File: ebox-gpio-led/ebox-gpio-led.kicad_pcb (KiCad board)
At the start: 2 copper layers, 45 x 75 mm, 26 parts, among them J1 xconch_pinheader_2x40, J2 xconch_pinsocket_2x40

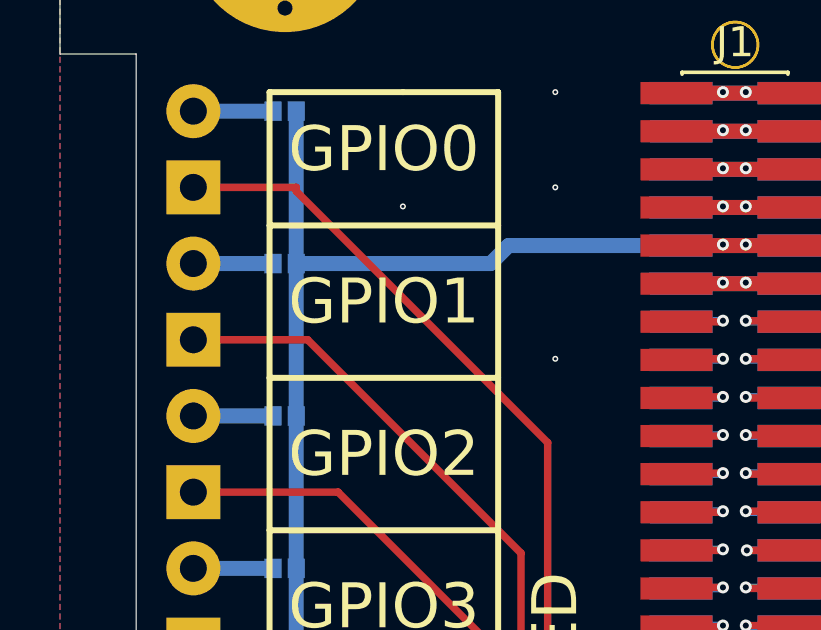
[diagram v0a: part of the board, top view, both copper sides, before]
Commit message: update some documents
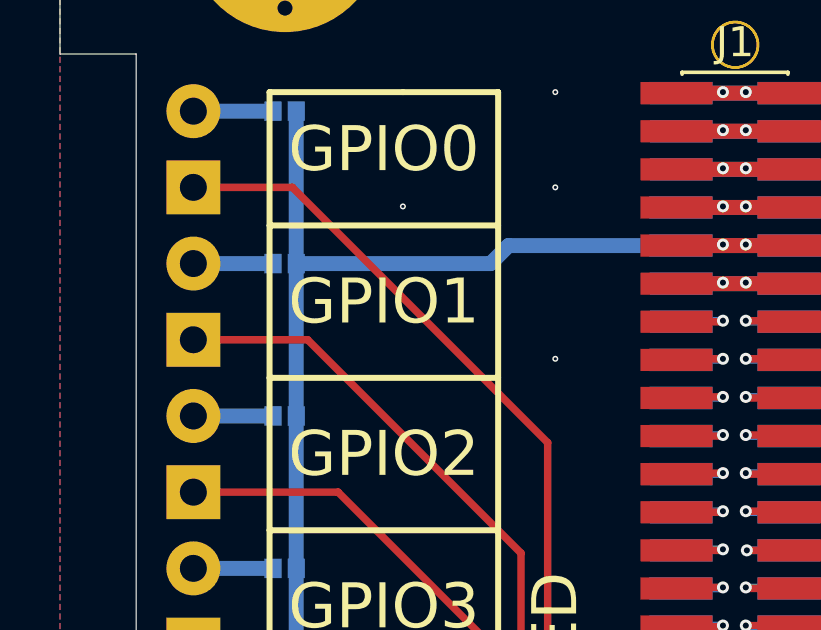
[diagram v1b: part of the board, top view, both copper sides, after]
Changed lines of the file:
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@@
     (thickness 1.6)
     (drawings 48)
-    (tracks 446)
+    (tracks 445)
     (zones 0)
     (modules 26)
@@
     (34 B.Paste user)
     (35 F.Paste user)
-    (36 B.SilkS user hide)
-    (37 F.SilkS user hide)
+    (36 B.SilkS user)
+    (37 F.SilkS user)
     (38 B.Mask user)
     (39 F.Mask user)
@@
     (46 B.CrtYd user)
     (47 F.CrtYd user)
-    (48 B.Fab user hide)
-    (49 F.Fab user hide)
+    (48 B.Fab user)
+    (49 F.Fab user)
   )
   (setup
-    (last_trace_width 0.125)
+    (last_trace_width 0.25)
     (user_trace_width 0.125)
     (user_trace_width 0.25)
@@
     (tags resistor)
     (attr smd)
-    (fp_text reference R1 (at -0.1205 -1.143 180) (layer B.SilkS)
+    (fp_text reference R1 (at 0.1205 1.143 180) (layer B.SilkS)
       (effects (font (size 1 1) (thickness 0.15)) (justify mirror))
     )
@@
     (tags resistor)
     (attr smd)
-    (fp_text reference R2 (at 0.0065 -1.143 180) (layer B.SilkS)
+    (fp_text reference R2 (at 0.0065 1.143 180) (layer B.SilkS)
       (effects (font (size 1 1) (thickness 0.15)) (justify mirror))
     )
@@
     (tags resistor)
     (attr smd)
-    (fp_text reference R3 (at 0 -1.143 180) (layer B.SilkS)
+    (fp_text reference R3 (at 0 1.143 180) (layer B.SilkS)
       (effects (font (size 1 1) (thickness 0.15)) (justify mirror))
     )
@@
     (tags resistor)
     (attr smd)
-    (fp_text reference R4 (at 0 -1.143 180) (layer B.SilkS)
+    (fp_text reference R4 (at 0 1.143 180) (layer B.SilkS)
       (effects (font (size 1 1) (thickness 0.15)) (justify mirror))
     )
@@
     (tags resistor)
     (attr smd)
-    (fp_text reference R5 (at 0 -1.143 180) (layer B.SilkS)
+    (fp_text reference R5 (at 0 1.143 180) (layer B.SilkS)
       (effects (font (size 1 1) (thickness 0.15)) (justify mirror))
     )
@@
     (tags resistor)
     (attr smd)
-    (fp_text reference R6 (at 0 -1.143 180) (layer B.SilkS)
+    (fp_text reference R6 (at 0.1205 1.143 180) (layer B.SilkS)
       (effects (font (size 1 1) (thickness 0.15)) (justify mirror))
     )
@@
     (tags resistor)
     (attr smd)
-    (fp_text reference R7 (at -0.1205 -1.143 180) (layer B.SilkS)
+    (fp_text reference R7 (at 0.1205 1.143 180) (layer B.SilkS)
       (effects (font (size 1 1) (thickness 0.15)) (justify mirror))
     )
@@
     (tags resistor)
     (attr smd)
-    (fp_text reference R8 (at 0.0065 -1.143 180) (layer B.SilkS)
+    (fp_text reference R8 (at 0.0065 1.143 180) (layer B.SilkS)
       (effects (font (size 1 1) (thickness 0.15)) (justify mirror))
     )
@@
     (tags resistor)
     (attr smd)
-    (fp_text reference R9 (at 0.0065 -1.143 180) (layer B.SilkS)
+    (fp_text reference R9 (at 0.0065 1.143 180) (layer B.SilkS)
       (effects (font (size 1 1) (thickness 0.15)) (justify mirror))
     )
@@
     (tags resistor)
     (attr smd)
-    (fp_text reference R10 (at -0.5015 -1.143 180) (layer B.SilkS)
+    (fp_text reference R10 (at 0.3745 1.143 180) (layer B.SilkS)
       (effects (font (size 1 1) (thickness 0.15)) (justify mirror))
     )
@@
   (segment (start 20.7 21.625) (end 22 21.625) (width 0.25) (layer B.Cu) (net 7) (status 10))
   (via (at 22.098 21.59) (size 0.4) (drill 0.2) (layers F.Cu B.Cu) (net 7))
-  (segment (start 4.445 15.875) (end 7.874 15.875) (width 0.25) (layer F.Cu) (net 33))
+  (segment (start 4.445 15.875) (end 7.747 15.875) (width 0.25) (layer F.Cu) (net 33))
+  (segment (start 7.747 15.875) (end 16.256 24.384) (width 0.25) (layer F.Cu) (net 33))
   (segment (start 16.256 24.384) (end 16.256 35.291) (width 0.25) (layer F.Cu) (net 33))
-  (segment (start 7.874 15.875) (end 7.874 16.002) (width 0.25) (layer F.Cu) (net 33))
-  (segment (start 7.874 16.002) (end 16.256 24.384) (width 0.25) (layer F.Cu) (net 33))
   (segment (start 16.256 35.291) (end 19.1 38.135) (width 0.25) (layer F.Cu) (net 33))
   (segment (start 19.1 38.135) (end 20.55 38.135) (width 0.25) (layer F.Cu) (net 33))
